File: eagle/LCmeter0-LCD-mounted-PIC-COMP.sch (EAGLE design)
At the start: 35 parts, among them IC1 PIC16F876A, J1 HD44780-4BITLCD44780-8P, J2 PIC-UART, J3 PIC-ICSP, J4 J4, J5 CONN-2P2P/V, J7 CONN-2P2P/V, K2 DS2Y, Q1 20MHz, SW1 PB-1P-1T, T1 BC547

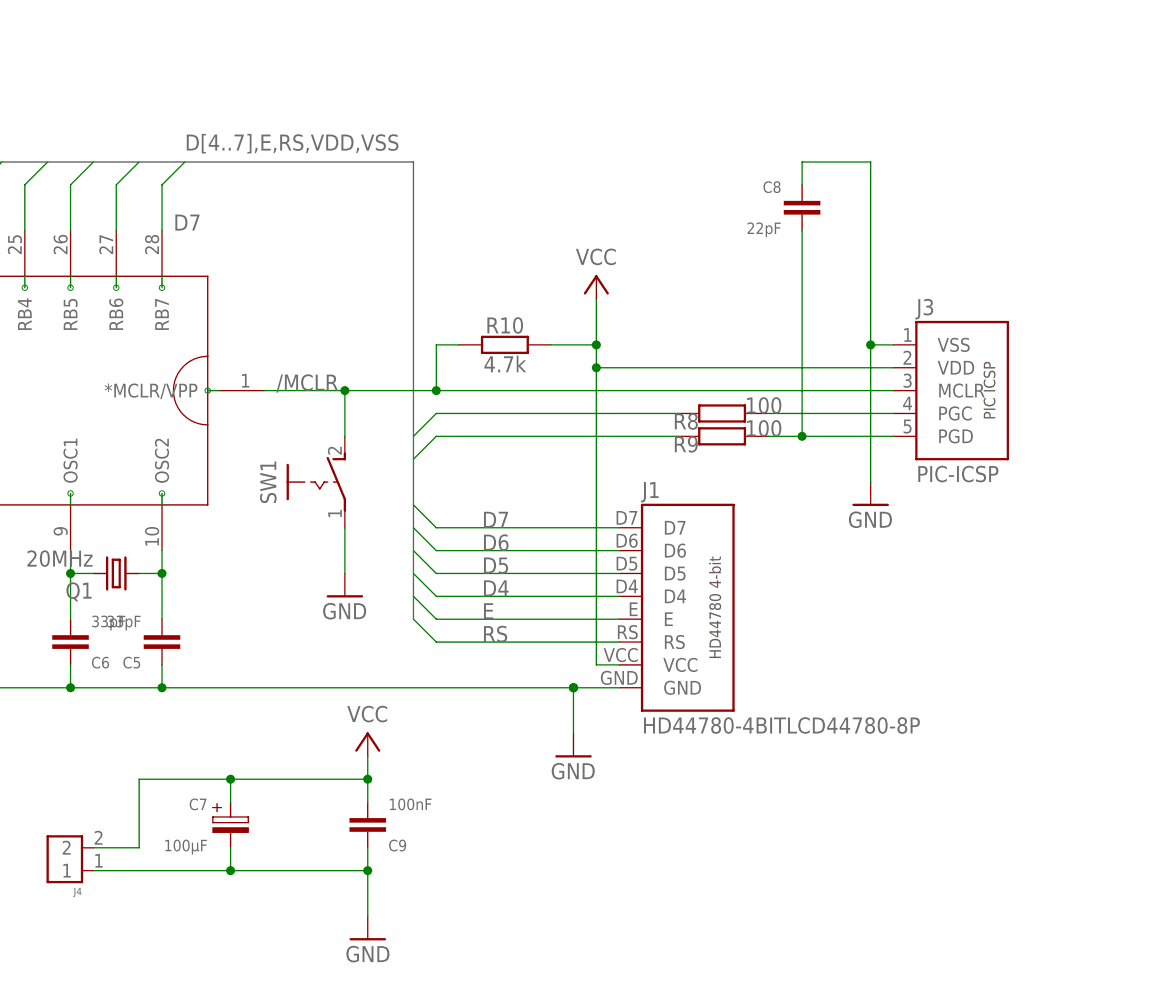
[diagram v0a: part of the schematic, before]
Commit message: ...
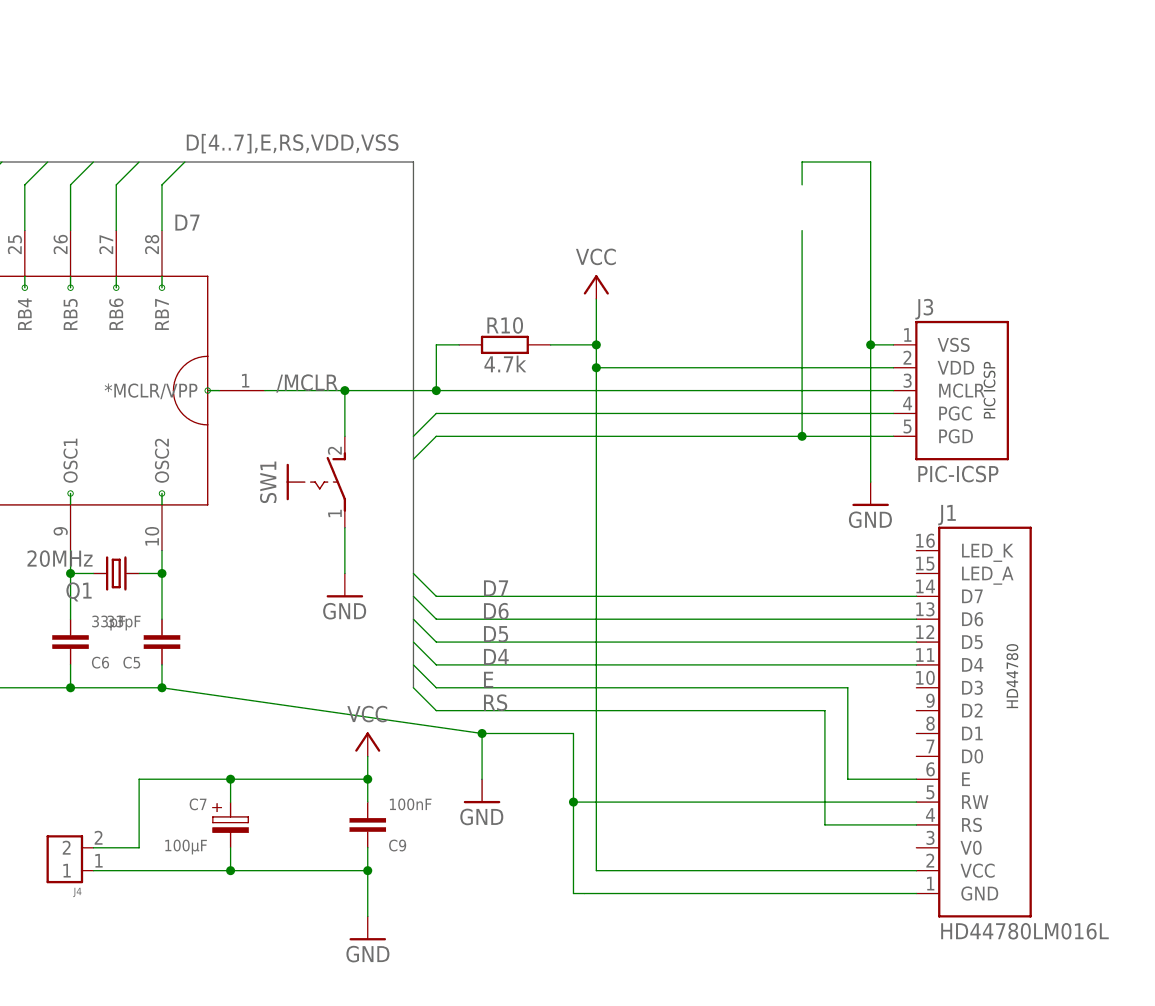
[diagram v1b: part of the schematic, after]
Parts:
- removed C8: 22pF, c:C050-020X036
- removed R8: 100, r:R0202/7-V
- removed R9: 100, r:R0202/5-V
- J1: value HD44780-4BITLCD44780-8P -> HD44780LM016L; device pinconn:HD44780-4BITLCD44780-8P -> lcd:HD44780LM016L
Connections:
- removed net PGC: J3.PGC, R8.1
- removed net PGD: C8.2, J3.PGD, R9.1
- net D6: now also J3.PGC; no longer R8.2
- net D7: now also J3.PGD; no longer R9.2
- net GND: now also J1.RW; no longer C8.1
